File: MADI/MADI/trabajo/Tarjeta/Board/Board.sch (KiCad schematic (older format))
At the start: 7 parts, among them J1 Conn_01x10_Female, J2 Conn_01x04_Female, J3 Conn_01x02_Female, J4 Conn_01x08_Female, J5 Conn_01x04_Female, J6 Conn_01x02_Female

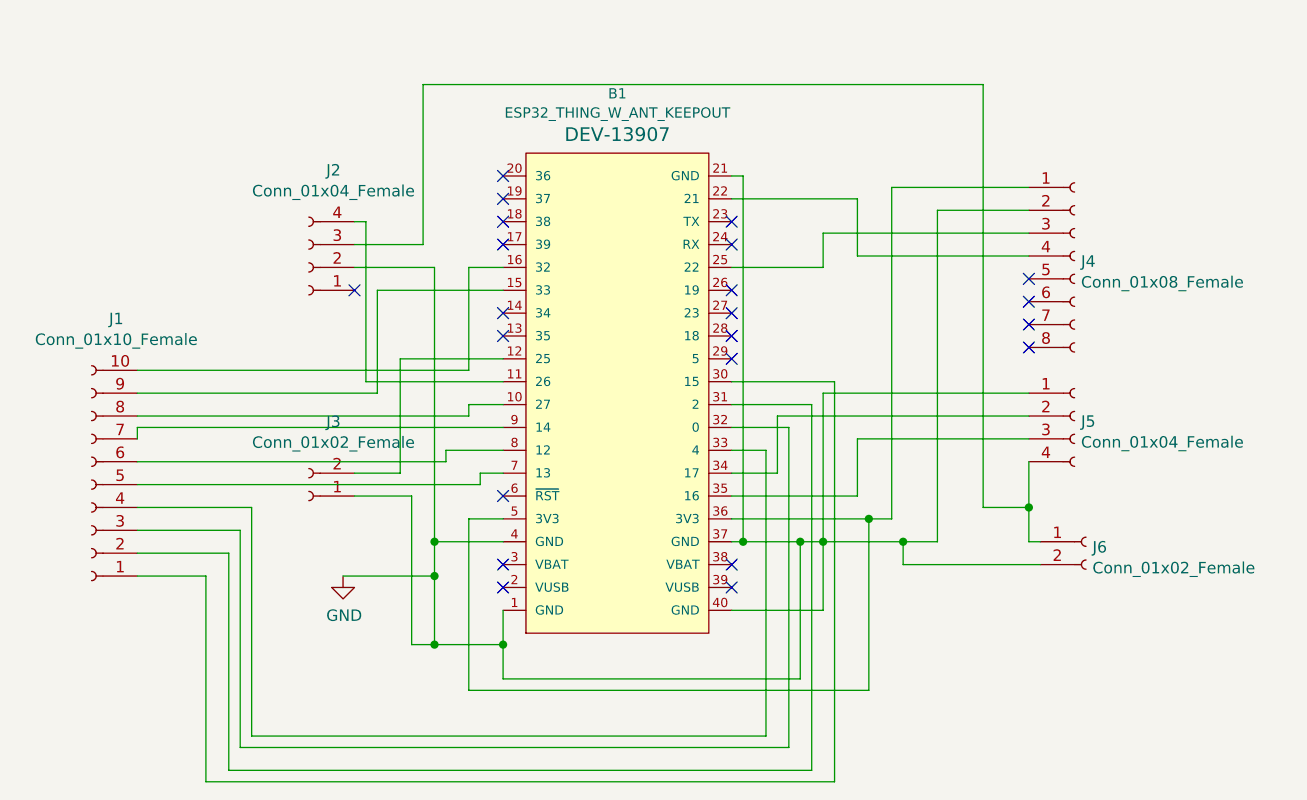
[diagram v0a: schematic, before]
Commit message: hola
Hola
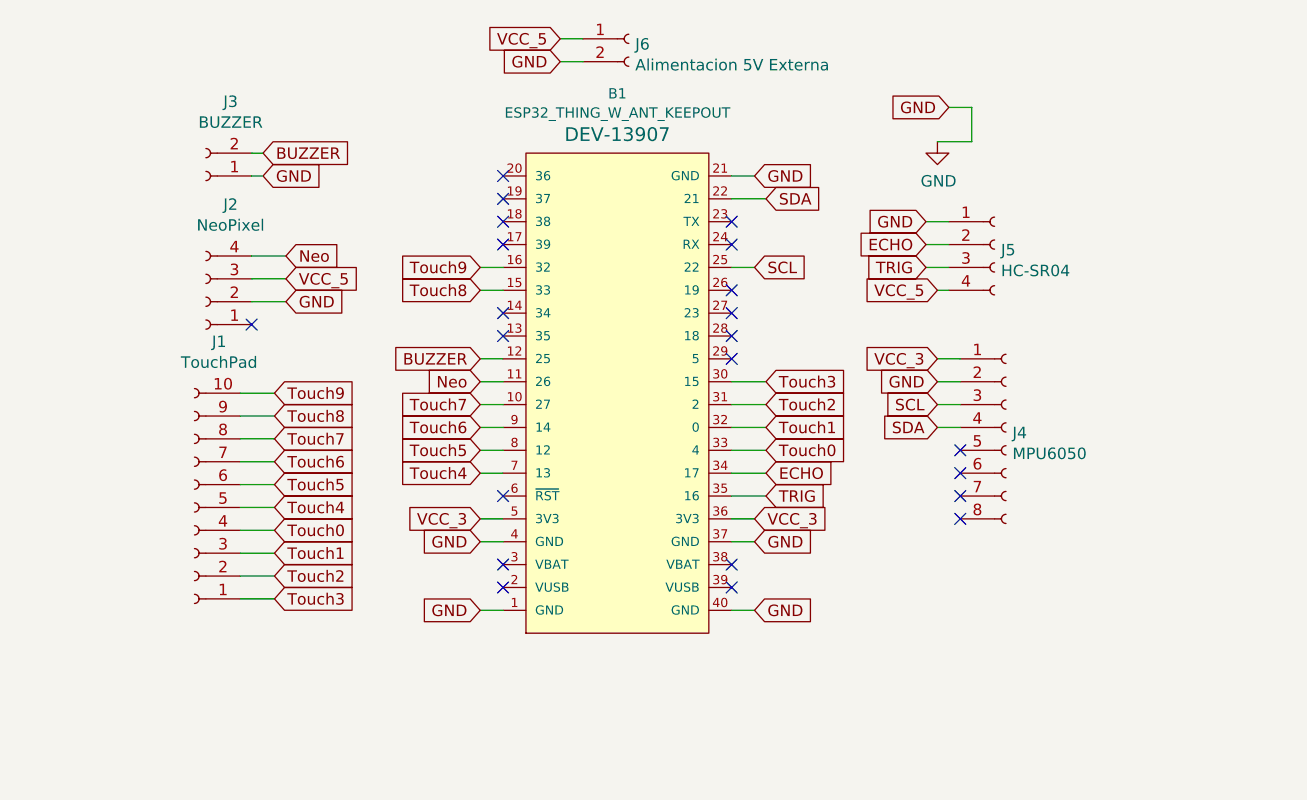
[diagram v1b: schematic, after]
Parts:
- J1: value Conn_01x10_Female -> TouchPad
- J2: value Conn_01x04_Female -> NeoPixel
- J3: value Conn_01x02_Female -> BUZZER
- J4: value Conn_01x08_Female -> MPU6050
- J5: value Conn_01x04_Female -> HC-SR04
- J6: value Conn_01x02_Female -> Alimentacion 5V Externa
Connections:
- net Touch7: now reaches B1.10 (27), J1.8 (Pin_8)
- net Neo: now reaches B1.11 (26), J2.4 (Pin_4)
- net BUZZER: now reaches B1.12 (25), J3.2 (Pin_2)
- net Touch8: now reaches B1.15 (33), J1.9 (Pin_9)
- net Touch9: now reaches B1.16 (32), J1.10 (Pin_10)
- net SDA: now reaches B1.22 (21), J4.4 (Pin_4)
- net SCL: now reaches B1.25 (22), J4.3 (Pin_3)
- net Touch3: now reaches B1.30 (15), J1.1 (Pin_1)
- net Touch2: now reaches B1.31 (2), J1.2 (Pin_2)
- net Touch1: now reaches B1.32 (0), J1.3 (Pin_3)
- net Touch0: now reaches B1.33 (4), J1.4 (Pin_4)
- net ECHO: now reaches B1.34 (17), J5.2 (Pin_2)
- net TRIG: now reaches B1.35 (16), J5.3 (Pin_3)
- net VCC_3: now reaches B1.36 (3V3), B1.5 (3V3), J4.1 (Pin_1)
- net Touch4: now reaches B1.7 (13), J1.5 (Pin_5)
- net Touch5: now reaches B1.8 (12), J1.6 (Pin_6)
- net Touch6: now reaches B1.9 (14), J1.7 (Pin_7)
- net VCC_5: now reaches J2.3 (Pin_3), J5.4 (Pin_4), J6.1 (Pin_1)
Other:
- moved on the sheet: J1, J2, J3, J4, J5, J6
